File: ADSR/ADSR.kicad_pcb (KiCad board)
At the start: 2 copper layers, 47 parts, among them J1 EuroPower, J2 GATE, J3 Hard Envelope, J4 Envelope, Q1 BC557, Q2 BC547, Q3 BC547, Q4 BC547, U1 LM741, U2 LM741, U3 LM741, U4 LM741, U5 LM741

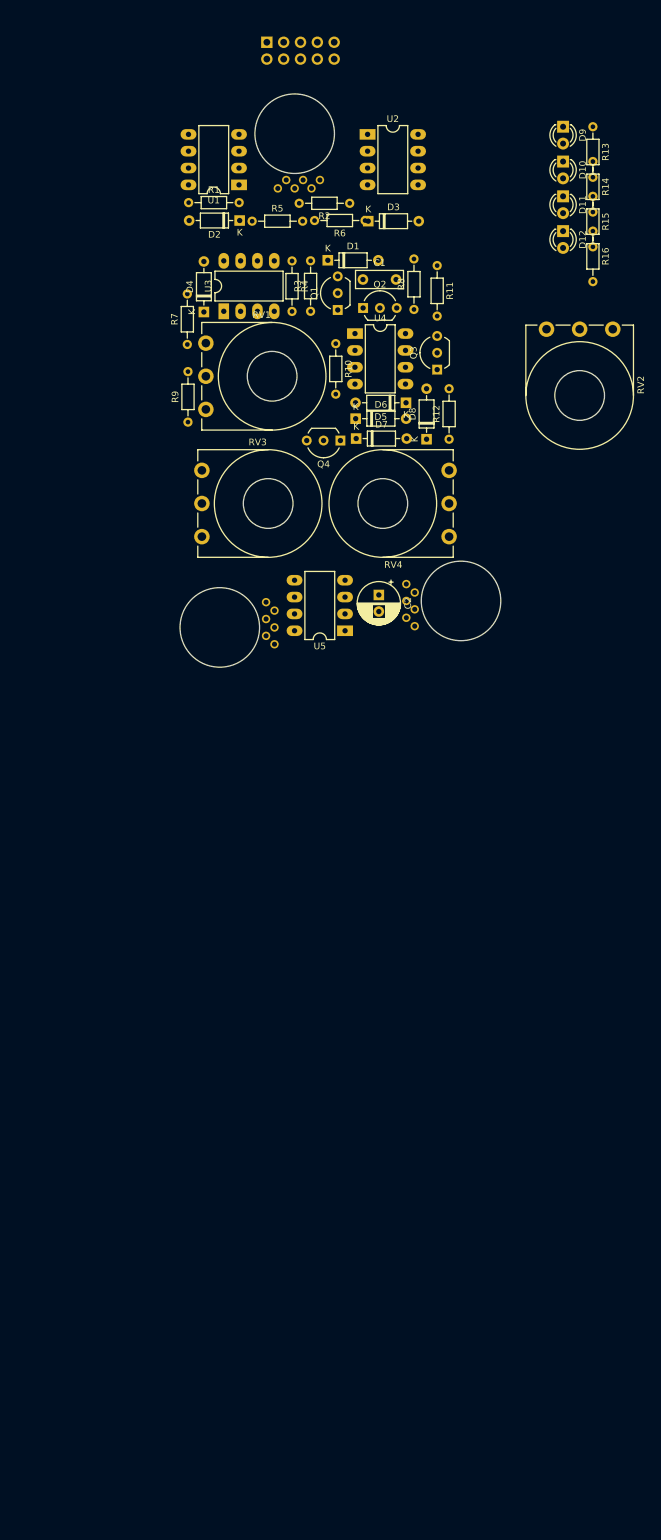
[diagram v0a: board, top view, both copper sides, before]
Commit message: Will it fits ?
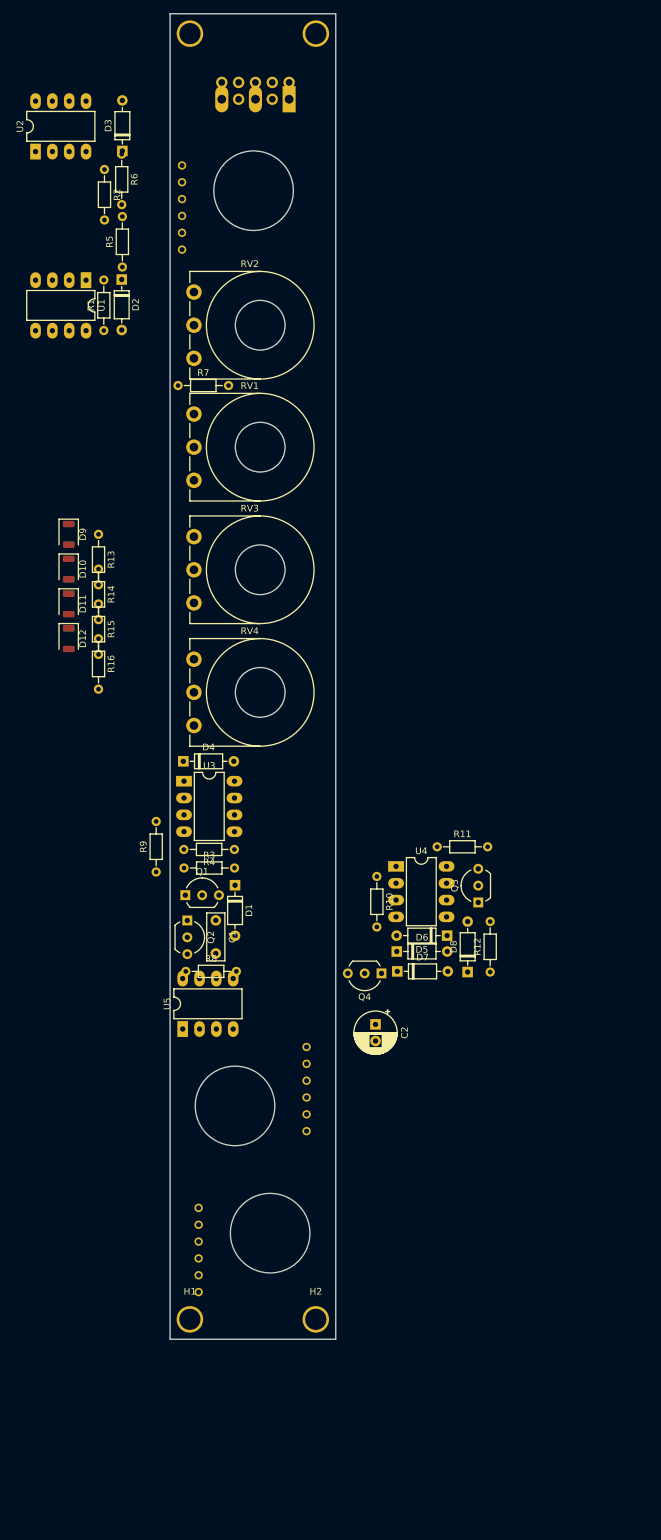
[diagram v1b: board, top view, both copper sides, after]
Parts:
- added H1: Mounting_Holes, Kosmo_panel:Kosmo_Panel_Dual_Mounting_Holes, F.Cu at (15.0, 209.0)
- added H2: Mounting_Holes, Kosmo_panel:Kosmo_Panel_Dual_Mounting_Holes, F.Cu at (34.0, 209.0)
- D10, D11, D12, D9: footprint LED_THT:LED_D3.0mm -> LED_SMD:LED_1206_3216Metric_ReverseMount_Hole1.8x2.4mm
- J1: footprint Connector_IDC:IDC-Header_2x05_P2.54mm_Vertical -> telec:EuroPower
- moved R8 105.6 mm to (14.4, 156.5), turned to 0 degrees
- moved J3 99.7 mm to (27.1, 196.0)
- moved C1 99.2 mm to (18.9, 148.8), turned to 270 degrees
- moved D10 96.7 mm to (-3.30, 95.8)
- moved D11 96.7 mm to (-3.30, 101.0)
- moved D12 96.7 mm to (-3.30, 106.3)
- moved D9 96.7 mm to (-3.30, 90.5)
- moved R13 96.7 mm to (1.20, 90.5)
- moved R14 96.7 mm to (1.20, 95.8)
- moved R15 96.7 mm to (1.20, 101.0)
- moved R16 96.7 mm to (1.20, 106.3)
- moved Q2 96.1 mm to (14.6, 148.8), turned to 270 degrees
- moved D1 95.3 mm to (21.8, 143.5), turned to 270 degrees
- moved Q1 91.2 mm to (14.3, 145.0), turned to 0 degrees
- moved R4 89.2 mm to (21.7, 138.1), turned to 180 degrees
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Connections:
- J1 pad 2: -12V -> GND
- J1 pad 3: GND -> +12V
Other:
- board outline added: 25 x 200 mm
- net class Default: clearance 0.2 -> 0.1524; trace_width 0.25 -> 0.1524; via_dia 0.8 -> 0.6858; via_drill 0.4 -> 0.3302
- rule trace_clearance: 0.2 -> 0.1524
- rule trace_min: 0.2 -> 0.1524
- rule via_min_drill: 0.3 -> 0.254
- rule via_min_size: 0.4 -> 0.508

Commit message: It fits !
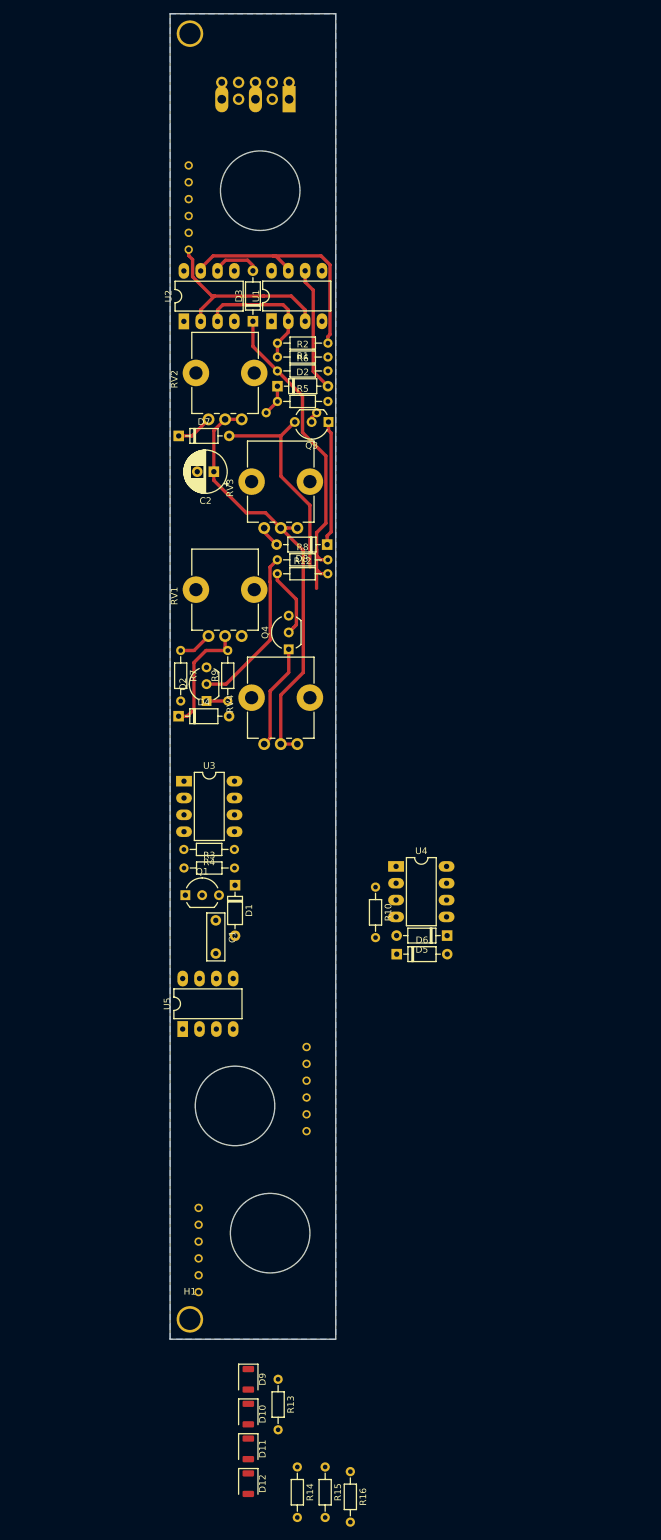
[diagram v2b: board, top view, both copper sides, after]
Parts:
- removed H2: Mounting_Holes, Kosmo_panel:Kosmo_Panel_Dual_Mounting_Holes
- R11: moved to B.Cu
- RV1, RV2, RV3, RV4: footprint Potentiometer_THT:Potentiometer_Piher_T-16L_Single_Vertical_Hole -> Potentiometer_THT:Potentiometer_Alps_RK09K_Single_Vertical
- moved R14 138.8 mm to (31.2, 231.3)
- moved R15 134.6 mm to (35.4, 231.3)
- moved R16 131.3 mm to (39.2, 232.0)
- moved D10 130.3 mm to (23.8, 223.3)
- moved D11 130.3 mm to (23.8, 228.6)
- moved D12 130.3 mm to (23.8, 233.8)
- moved D9 130.3 mm to (23.8, 218.1)
- moved R13 130.3 mm to (28.3, 218.1)
- moved D7 87.3 mm to (13.3, 75.7)
- moved C2 86.9 mm to (18.6, 81.1), turned to 180 degrees
- moved Q3 75.9 mm to (35.9, 73.6), turned to 180 degrees
- moved R11 70.4 mm to (26.5, 72.2)
- moved R12 68.1 mm to (28.2, 96.5), turned to 0 degrees
- moved D8 67.9 mm to (35.7, 92.1), turned to 180 degrees
- moved R8 63.6 mm to (28.2, 94.4)
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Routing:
- net /Cap: track 0.00 -> 66.1 mm
- net /~IN: track 0.00 -> 50.0 mm
- net +12V: track 0.00 -> 36.6 mm
- net /Hard: track 0.00 -> 32.4 mm
- net /GATE: track 0.00 -> 29.8 mm
- net Net-(Q2-Pad2): track 0.00 -> 24.9 mm
- net Net-(R1-Pad2): track 0.00 -> 20.8 mm
- net Net-(D8-Pad1): track 0.00 -> 18.9 mm
- net Net-(D2-Pad2): track 0.00 -> 18.8 mm
- net Net-(D4-Pad1): track 0.00 -> 18.0 mm
- net Net-(Q4-Pad1): track 0.00 -> 15.8 mm
- net Net-(Q4-Pad2): track 0.00 -> 10.5 mm
- net Net-(D3-Pad2): track 0.00 -> 7.35 mm
- net Net-(D7-Pad1): track 0.00 -> 5.54 mm
- net Net-(R7-Pad1): track 0.00 -> 5.10 mm
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- added copper zone on B.Cu, net GND

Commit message: Now the power lines...
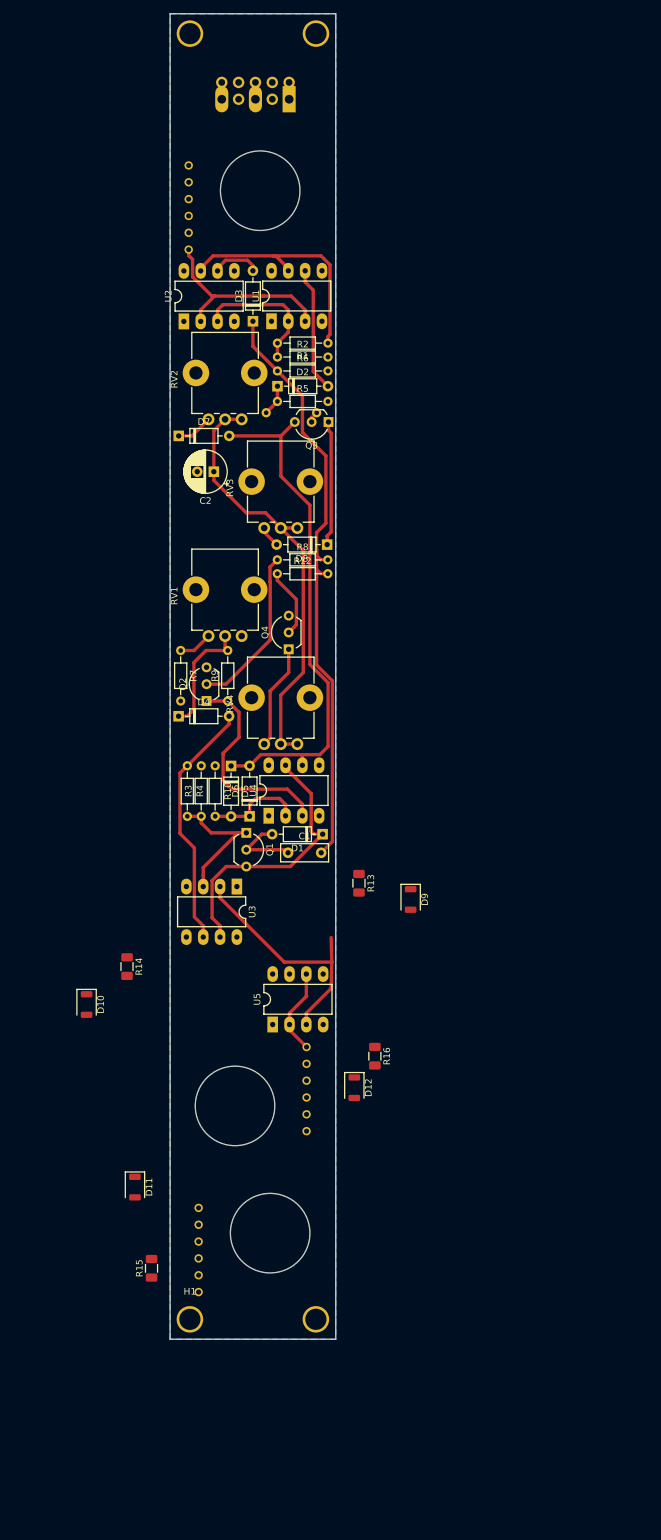
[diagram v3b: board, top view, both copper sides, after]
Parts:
- added H2: Mounting_Holes, Kosmo_panel:Kosmo_Panel_Dual_Mounting_Holes, F.Cu at (34.0, 209.0)
- R13, R14: footprint Resistor_THT:R_Axial_DIN0204_L3.6mm_D1.6mm_P7.62mm_Horizontal -> Resistor_SMD:R_1206_3216Metric
- R15, R16: value 1k5 -> 2k2; footprint Resistor_THT:R_Axial_DIN0204_L3.6mm_D1.6mm_P7.62mm_Horizontal -> Resistor_SMD:R_1206_3216Metric
- moved R14 79.8 mm to (5.50, 155.8)
- moved D9 76.4 mm to (48.3, 145.7)
- moved R13 75.8 mm to (40.5, 143.2)
- moved D10 66.4 mm to (-0.60, 161.5)
- moved R16 62.8 mm to (42.9, 169.3)
- moved D12 61.9 mm to (39.8, 174.1)
- moved D11 43.0 mm to (6.70, 189.1)
- moved D5 41.5 mm to (21.2, 125.5), turned to 270 degrees
- moved R15 39.8 mm to (9.20, 201.3), turned to 90 degrees
- moved D6 30.4 mm to (24.0, 133.1), turned to 90 degrees
- moved R10 30.3 mm to (18.8, 125.5)
- moved U4 20.7 mm to (26.9, 133.0), turned to 90 degrees
- moved U3 17.8 mm to (22.1, 143.7), turned to 270 degrees
- moved D1 15.3 mm to (35.0, 135.8), turned to 180 degrees
- moved C1 14.9 mm to (29.8, 138.6), turned to 0 degrees
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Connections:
- D9 pad 1: GND -> Net-(D9-Pad1)
- D9 pad 2: Net-(D9-Pad2) -> GND
- R13 pad 1: /IN -> /~IN
- R13 pad 2: Net-(D9-Pad2) -> Net-(D9-Pad1)
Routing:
- net /Hard: track 32.4 -> 78.1 mm
- net +12V: track 36.6 -> 78.7 mm
- net /~IN: track 50.0 -> 91.6 mm
- net /Triggered: track 0.00 -> 37.8 mm
- net /Cap: track 66.1 -> 103.4 mm
- net Net-(Q2-Pad1): track 3.20 -> 32.1 mm
- net Net-(Q1-Pad1): track 0.00 -> 20.8 mm
- net Net-(D5-Pad2): track 0.00 -> 14.9 mm
- net /Envelope: track 0.00 -> 13.2 mm
- net Net-(C1-Pad1): track 0.00 -> 11.4 mm
